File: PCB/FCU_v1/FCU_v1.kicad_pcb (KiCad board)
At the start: 4 copper layers, 57.6 x 60.8 mm, 96 parts, among them IC1 BMM350, IC2 TPS7A2018PDBVR, IC3 ESP32-C3-MINI-1-N4X, J1 Conn_01x04_Pin, J10 Conn_01x04_Pin, J11 USB_C_Receptacle_USB2.0_16P, J3 Conn_01x05_Pin, J5 Conn_01x04_Pin, J6 Conn_01x04_Pin, J7 Conn_01x04_Pin, J8 Conn_01x04_Pin, J9 Conn_01x04_Pin, U1 TPS62A02APDDCR, U10 SN65HVD232, U11 STM32G473RETx, U2 BMP581, U3 W25Q128JVSIM, U4 BMI088, U8 USBLC6-2SC6, Y2 16MHz

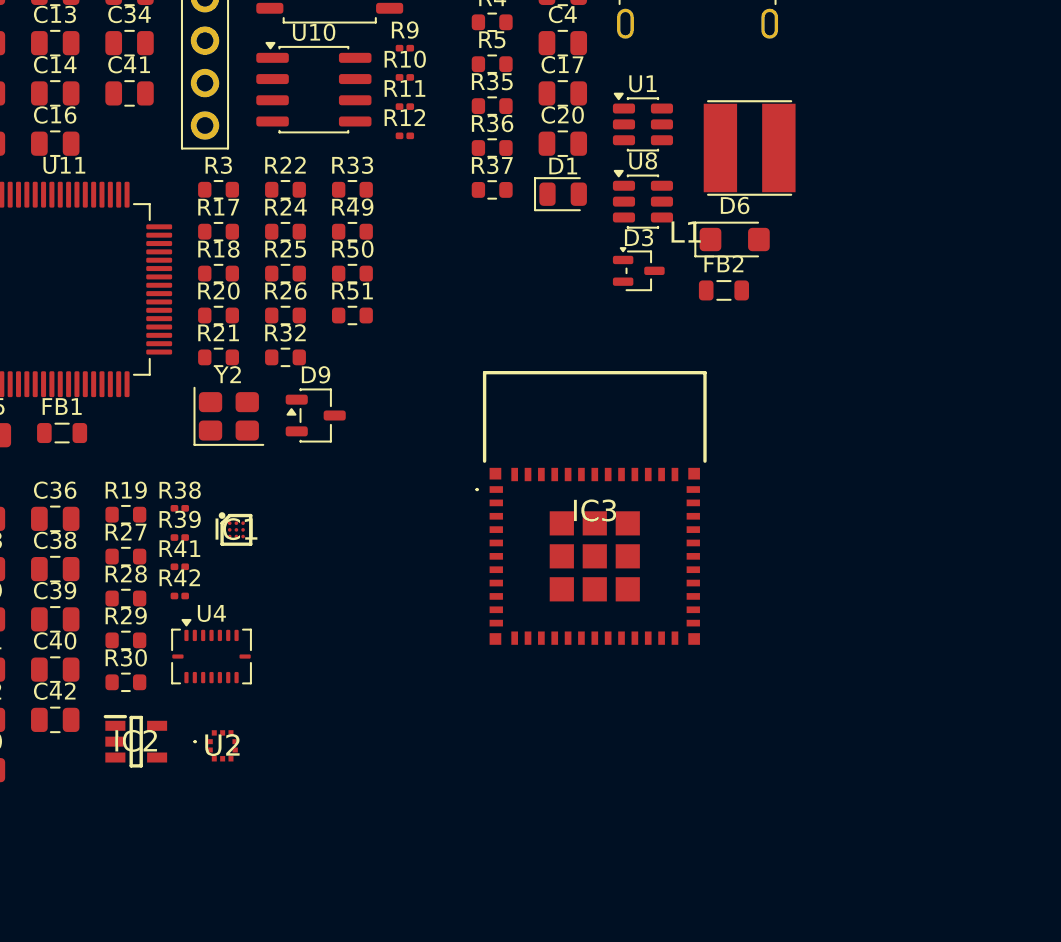
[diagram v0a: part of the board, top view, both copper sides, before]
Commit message: Repaired library
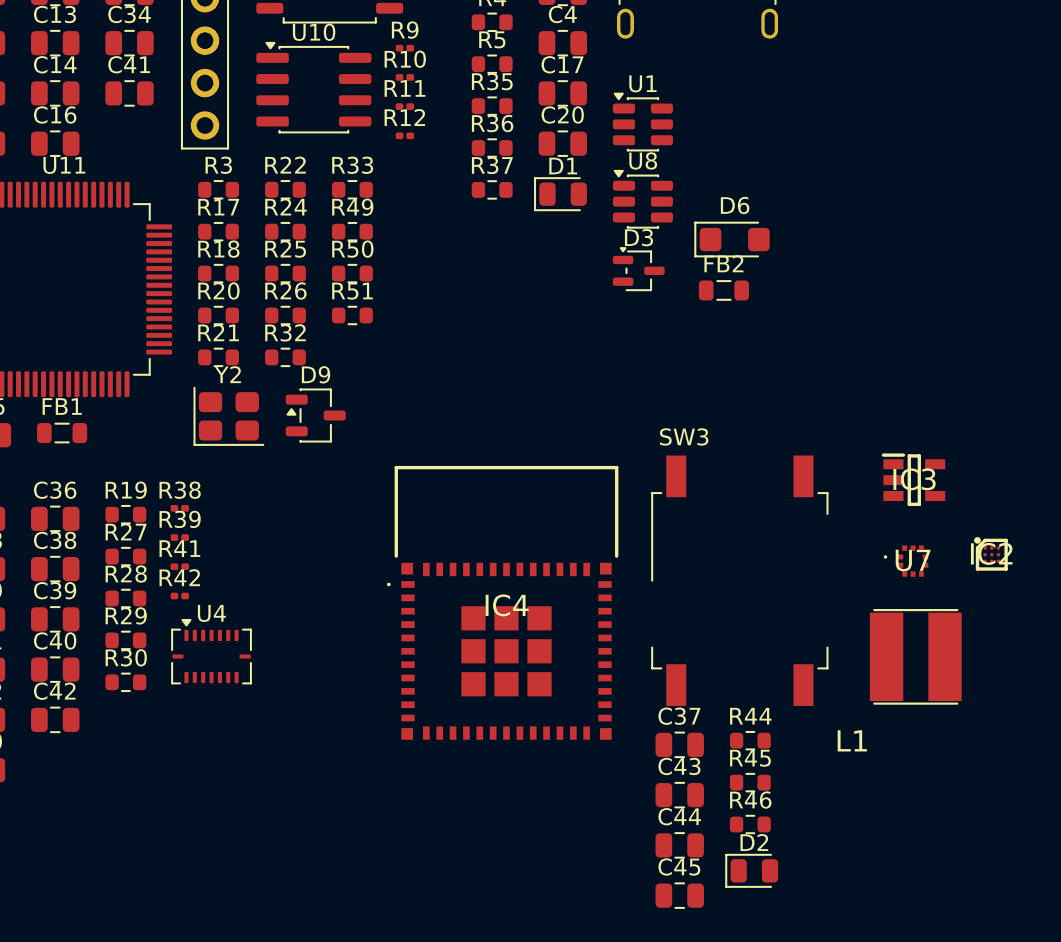
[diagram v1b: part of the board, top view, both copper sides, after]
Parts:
- removed IC1: BMM350, SamacSys_Parts:BGA9C40P3X3_128X128X54
- removed U2: BMP581, SamacSys_Parts:BMP581
- added C37: 10u, Capacitor_SMD:C_0805_2012Metric, F.Cu at (221.4, 125.0)
- added C43: 100n, Capacitor_SMD:C_0805_2012Metric, F.Cu at (221.4, 128.0)
- added C44: 1u, Capacitor_SMD:C_0805_2012Metric, F.Cu at (221.4, 131.0)
- added C45: 100n, Capacitor_SMD:C_0805_2012Metric, F.Cu at (221.4, 134.0)
- added D2: LED, LED_SMD:LED_0805_2012Metric, F.Cu at (225.9, 132.5)
- added IC4: ESP32-C3-MINI-1-N4X, SamacSys_Parts:ESP32C3MINI1N4X, F.Cu at (211.1, 116.7)
- added R44: 10k, Resistor_SMD:R_0603_1608Metric, F.Cu at (225.7, 124.7)
- added R45: 10k, Resistor_SMD:R_0603_1608Metric, F.Cu at (225.7, 127.2)
- added R46: 2k, Resistor_SMD:R_0603_1608Metric, F.Cu at (225.7, 129.7)
- added SW3: SW_MEC_5G, Button_Switch_SMD:SW_MEC_5GSH9, F.Cu at (225.0, 115.1)
- added U7: BMP581, SamacSys_Parts:BMP581, F.Cu at (235.4, 114.0)
- IC2: value TPS7A2018PDBVR -> BMM350; footprint SamacSys_Parts:SOT95P280X145-5N -> SamacSys_Parts:BGA9C40P3X3_128X128X54
- IC3: value ESP32-C3-MINI-1-N4X -> TPS7A2018PDBVR; footprint SamacSys_Parts:ESP32C3MINI1N4X -> SamacSys_Parts:SOT95P280X145-5N
- moved IC2 52.5 mm to (240.1, 113.6)
- moved L1 32.1 mm to (235.6, 119.7)
- moved IC3 19.2 mm to (235.5, 109.1)
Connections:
- net STM_VDDA renamed +3.3VA
- C1 pad 1: +3.3V -> STM_VDD
- C11 pad 1: 3V3_FCU -> STM_VDD
- C14 pad 1: 3V3_FCU -> STM_VDD
- C18 pad 1: Net-(IC1-VDD) -> Net-(IC2-VDD)
- C19 pad 1: +3.3V -> STM_VDD
- C21 pad 1: +3.3V -> STM_VDD
- C22 pad 1: +3.3V -> STM_VDD
- C3 pad 1: Net-(IC1-CRST) -> Net-(IC2-CRST)
- C30 pad 1: +3.3V -> STM_VDD
- C31 pad 1: +3.3V -> STM_VDD
- C33 pad 1: +3.3V -> STM_VDD
- C34 pad 1: +3.3V -> STM_VDD
- C36 pad 1: Net-(IC1-VDD) -> Net-(IC2-VDD)
- C38 pad 1: +3.3V -> STM_VDD
- C39 pad 1: +3.3V -> STM_VDD
- C40 pad 1: +3.3V -> STM_VDD
- C42 pad 1: +3.3V -> STM_VDD
- C5 pad 1: 3V3_FCU -> STM_VDD
- C6 pad 1: 3V3_FCU -> STM_VDD
- C7 pad 1: 3V3_FCU -> STM_VDD
- C8 pad 1: 3V3_FCU -> STM_VDD
- C9 pad 1: 3V3_FCU -> STM_VDD
- FB1 pad 2: 3V3_FCU -> STM_VDD
- IC3 pad 1: GND -> STM_VDD
- IC3 pad 3: unconnected-(IC3-3V3-Pad3) -> STM_VDD
- IC3 pad 5: unconnected-(IC3-IO2-Pad5) -> Net-(IC2-VDD)
- J3 pad 1: +3.3V -> STM_VDD
- L1 pad 2: +3.3V -> STM_VDD
- R1 pad 1: +3.3V -> STM_VDD
- R12 pad 2: +3.3V -> STM_VDD
- R17 pad 1: I2C_SCL -> STM_VDD
- R17 pad 2: 3V3_FCU -> I2C_SCL
- R18 pad 1: I2C_SDA -> STM_VDD
- R18 pad 2: 3V3_FCU -> I2C_SDA
- R2 pad 1: +3.3V -> STM_VDD
- R38 pad 1: Net-(IC1-ADSEL) -> Net-(IC2-ADSEL)
- R39 pad 1: +3.3V -> STM_VDD
- R39 pad 2: Net-(IC1-ADSEL) -> Net-(IC2-ADSEL)
- R41 pad 1: +3.3V -> STM_VDD
- R9 pad 2: +3.3V -> STM_VDD
- U10 pad 3: +3.3V -> STM_VDD
- U11 pad 1: 3V3_FCU -> STM_VDD
- U11 pad 16: 3V3_FCU -> STM_VDD
- U11 pad 32: 3V3_FCU -> STM_VDD
- U11 pad 48: 3V3_FCU -> STM_VDD
- U11 pad 64: 3V3_FCU -> STM_VDD
- U3 pad 8: +3.3V -> STM_VDD
- U4 pad 11: +3.3V -> STM_VDD
- U4 pad 3: +3.3V -> STM_VDD
